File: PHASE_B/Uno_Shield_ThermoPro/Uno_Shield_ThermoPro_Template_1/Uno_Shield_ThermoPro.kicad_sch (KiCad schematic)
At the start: 20 parts, among them J1 Power, J2 Digital/PWM, J3 Analog, J4 Digital/PWM, J5 CONN_GYRO, J6 CONN_DISPLAY, J7 CONN_TEMP, SW1 SW_SPST, SW2 SW_SPST, SW3 SW_SPST, SW4 SW_SPST, SW5 SW_SPST

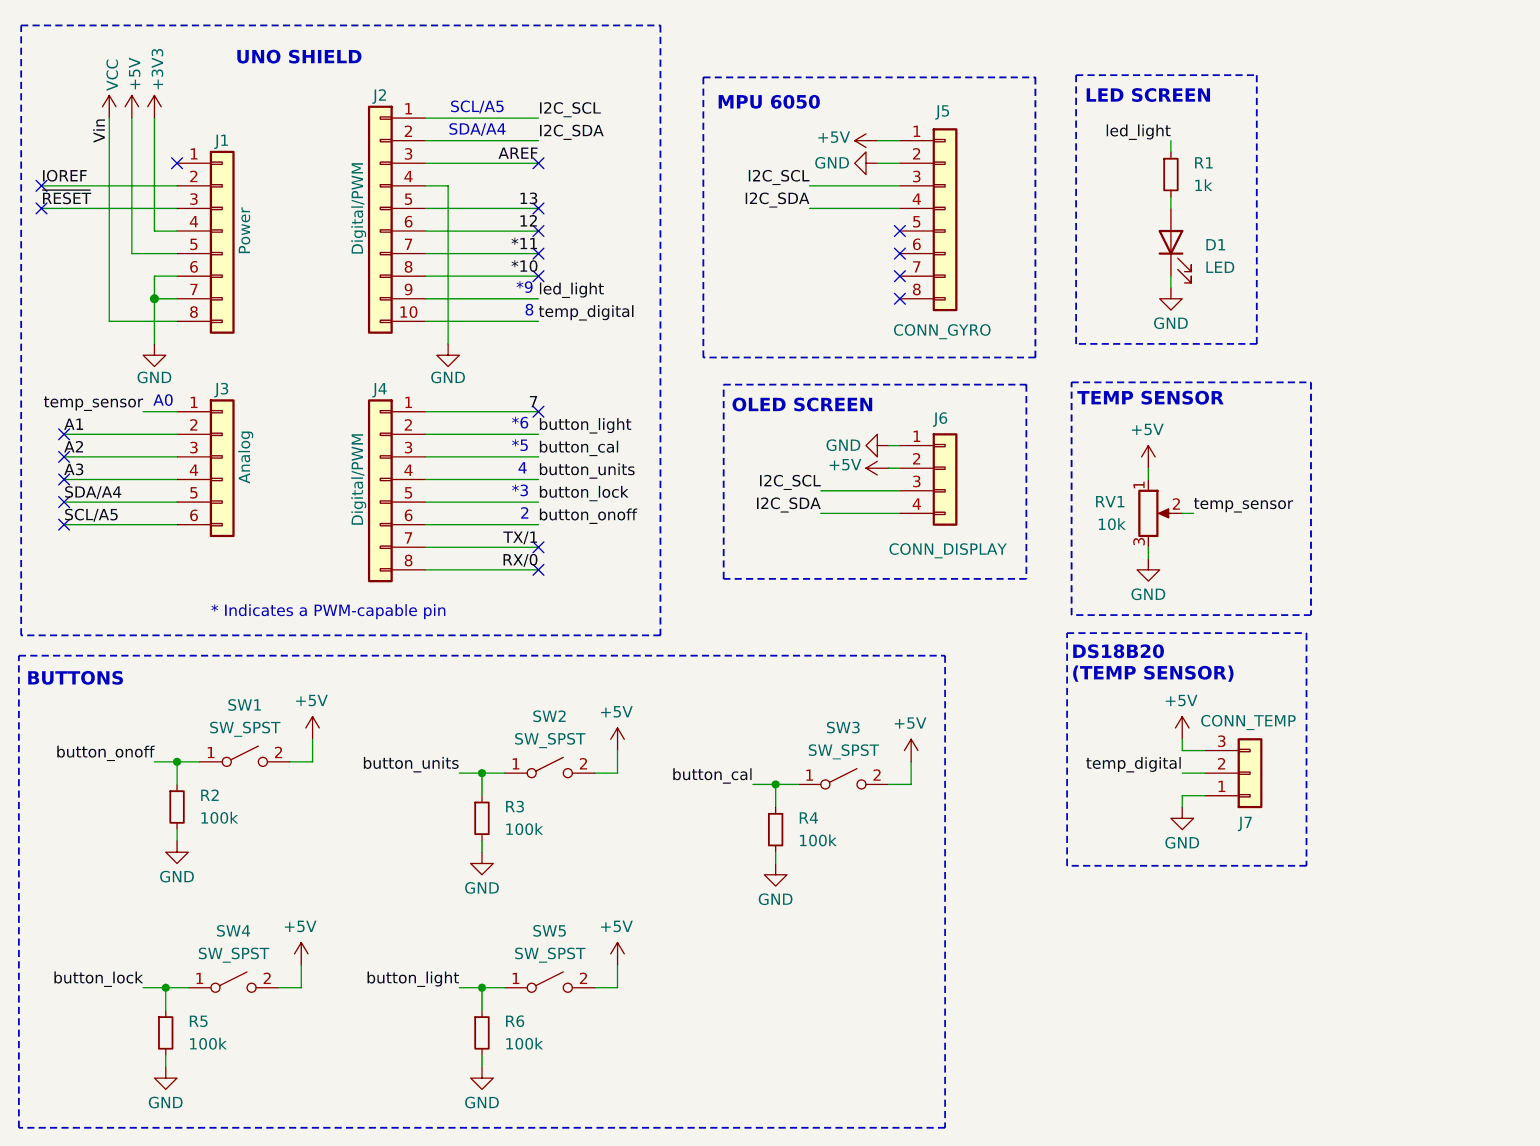
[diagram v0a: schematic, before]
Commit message: update
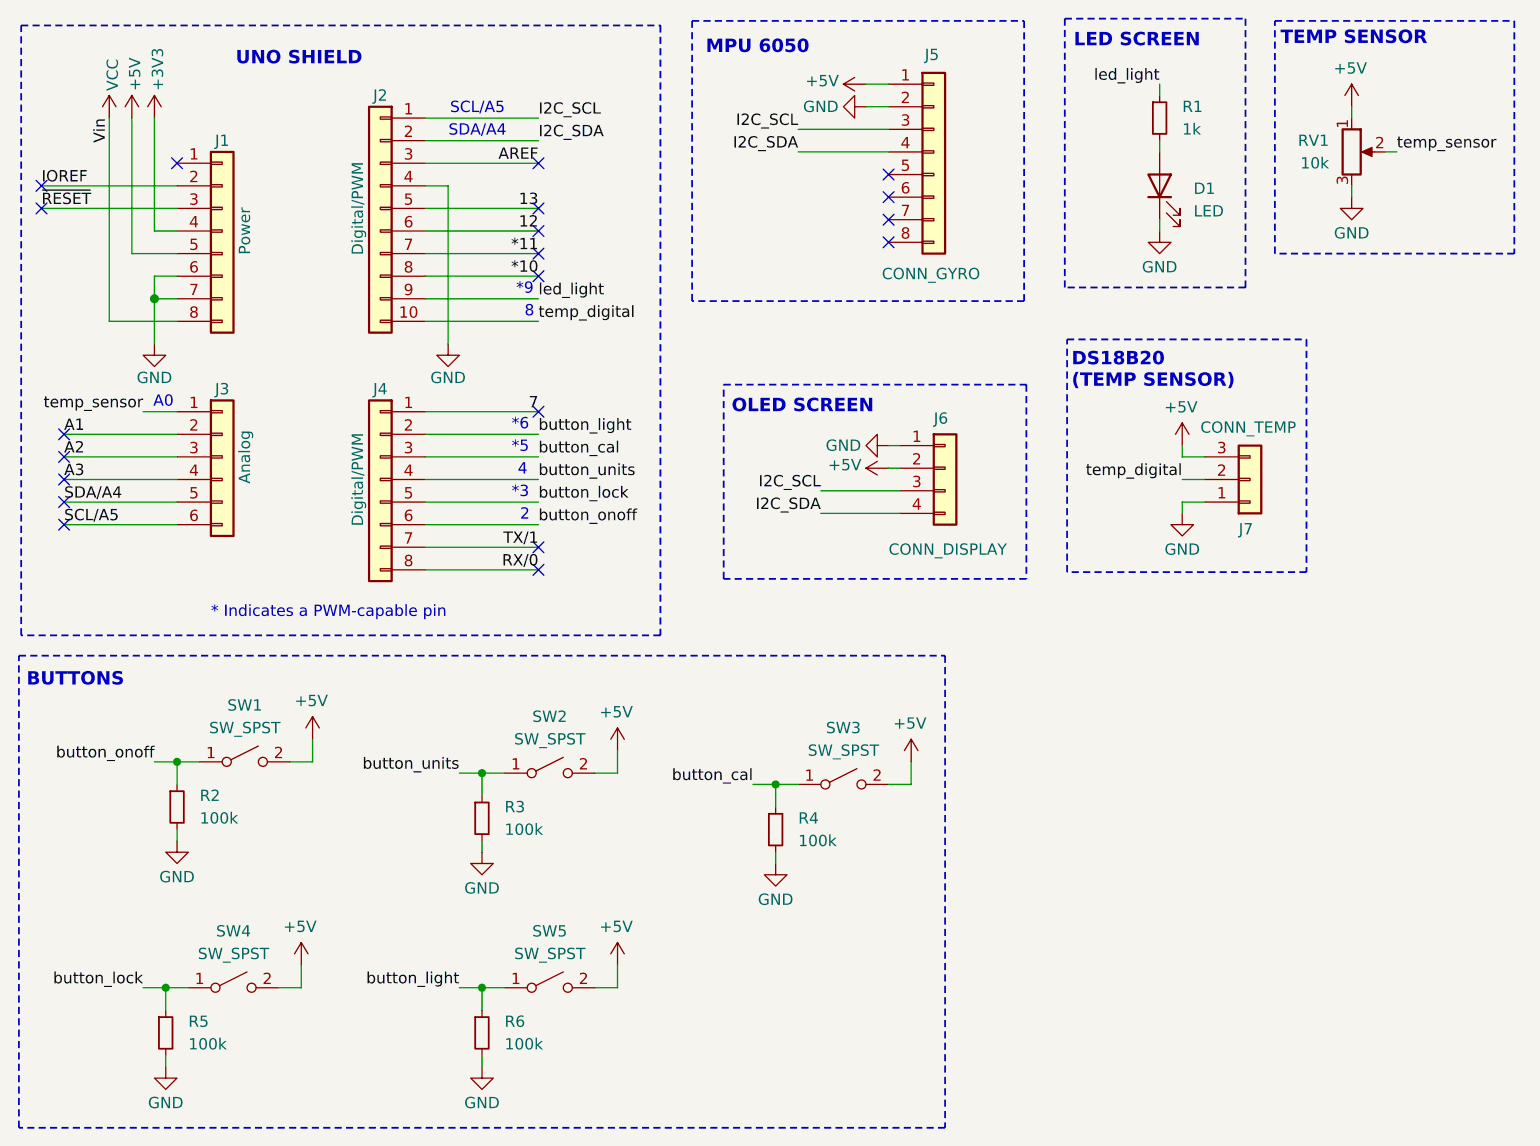
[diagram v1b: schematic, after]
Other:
- company: Goncalo Martins -> Luciano Henriquez
- moved on the sheet: D1, J5, J7, R1, RV1
